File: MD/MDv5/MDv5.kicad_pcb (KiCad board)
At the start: 2 copper layers, 59.3 x 78.1 mm, 46 parts, among them J1 XT60PW-M, J2 XT60PW-M, J3 XT30PW-M, J4 XT30PW-M

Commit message: IRLB3813,L7805CV,L7812CV,74HC08N,78HC14NをSMDにして回路図完成
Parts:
- removed C1: 330μF, Capacitor_THT:CP_Radial_D8.0mm_P3.50mm
- removed C10, C11: 1.5μF, Library:C_Disc_D11.0mm_W5.0mm_P5.0mm_kai
- removed C2, C4, C6, C7, C8, C9: 0.1μF, Library:C_Disc_D11.0mm_W5.0mm_P5.0mm_kai
- removed C3, C5: 33μF, Capacitor_THT:CP_Radial_D5.0mm_P2.00mm
- removed D1: PWM_IN, LED_THT:LED_D5.0mm
- removed D2: 5V/2, LED_THT:LED_D5.0mm
- removed D3: 12V, LED_THT:LED_D5.0mm
- removed D4, D5: 1N4148DO35-7, Diode_THT:D_DO-35_SOD27_P7.62mm_Horizontal
- removed FET1, FET2, FET3, FET4: IRLB3813PBF, footprints:PG-TO220-3_INF
- removed IC1_NOT1, IC2_AND1: ~, Package_DIP:DIP-14_W7.62mm
- removed IC3, IC4, TLP2630: ~, Package_DIP:DIP-8_W7.62mm
- removed J1, J2: XT60PW-M, XT60-M:AMASS_XT60PW-M
- removed J3, J4: XT30PW-M, XT60-M:AMASS_XT30PW-M
- removed R1, R6, R7: 330Ω, Library:R_Axial_DIN0207_L6.3mm_D2.5mm_P10.16mm_Horizontal_kai
- removed R10, R11, R8, R9: 10kΩ, Library:R_Axial_DIN0207_L6.3mm_D2.5mm_P10.16mm_Horizontal_kai
- removed R2, R3, R4, R5: 200Ω, Library:R_Axial_DIN0207_L6.3mm_D2.5mm_P10.16mm_Horizontal_kai
- removed REF** (x4): MountingHole_3.2mm_M3, MountingHole:MountingHole_3.2mm_M3
- removed REFG5V1: L7805, footprints:PG-TO220-3_INF
- removed REG12V1: L7812, footprints:PG-TO220-3_INF
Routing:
- net +5V/2: track 126.3 -> 0.00 mm
- net GATE2: track 99.0 -> 0.00 mm, vias 4 -> 0
- net GND1: track 78.7 -> 0.00 mm, vias 1 -> 0
- net +12V: track 73.1 -> 0.00 mm
- net PWM_IN: track 67.8 -> 0.00 mm, vias 1 -> 0
- net GATE1: track 62.0 -> 0.00 mm
- net DIGITAL_IN: track 56.9 -> 0.00 mm, vias 1 -> 0
- net Net-(FET1-G): track 43.7 -> 0.00 mm, vias 2 -> 0
- net MOUT1: track 39.3 -> 0.00 mm, vias 2 -> 0
- net Net-(FET2-G): track 38.0 -> 0.00 mm, vias 6 -> 0
- net PWM_NOT: track 36.8 -> 0.00 mm, vias 3 -> 0
- net PWM1: track 31.6 -> 0.00 mm
- net Net-(D2-A): track 26.1 -> 0.00 mm
- net DIGITAL: track 25.7 -> 0.00 mm, vias 2 -> 0
- net DIGITAL_NOT: track 24.3 -> 0.00 mm, vias 1 -> 0
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- removed copper zone on B.Cu, net +24V
- removed copper zone on B.Cu, net GND2
- removed copper zone on F.Cu, net GND2
- removed copper zone on F.Cu, net MOUT1
- removed copper zone on F.Cu, net MOUT2
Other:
- board outline removed
- board text removed: "24V24V24V"
- board text removed: "DIGITAL_IN"
- board text removed: "GND1"
- board text removed: "GND2"
- board text removed: "MOUT1"
- board text removed: "MOUT2"
- board text removed: "PWM_IN"

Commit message: とりあえず配置
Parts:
- added C1: 330μF, Capacitor_THT:CP_Radial_D8.0mm_P3.50mm, F.Cu at (151.9, 100.6)
- added C10: 1.5μF, Library:C_Disc_D11.0mm_W5.0mm_P5.0mm_kai, F.Cu at (142.9, 77.2)
- added C11: 1.5μF, Library:C_Disc_D11.0mm_W5.0mm_P5.0mm_kai, F.Cu at (158.1, 76.9)
- added C2: 0.1μF, Library:C_Disc_D11.0mm_W5.0mm_P5.0mm_kai, F.Cu at (161.8, 106.7)
- added C3: 33μF, Capacitor_THT:CP_Radial_D5.0mm_P2.00mm, F.Cu at (162.9, 97.4)
- added C4: 0.1μF, Library:C_Disc_D11.0mm_W5.0mm_P5.0mm_kai, F.Cu at (151.2, 88.0)
- added C5: 33μF, Capacitor_THT:CP_Radial_D5.0mm_P2.00mm, F.Cu at (162.9, 90.9)
- added C6: 0.1μF, Library:C_Disc_D11.0mm_W5.0mm_P5.0mm_kai, F.Cu at (163.1, 86.0)
- added C7: 0.1μF, Library:C_Disc_D11.0mm_W5.0mm_P5.0mm_kai, F.Cu at (152.7, 69.3)
- added C8: 0.1μF, Library:C_Disc_D11.0mm_W5.0mm_P5.0mm_kai, F.Cu at (138.5, 69.3)
- added C9: 0.1μF, Library:C_Disc_D11.0mm_W5.0mm_P5.0mm_kai, F.Cu at (150.8, 53.7)
- added D1: PWM_IN, LED_THT:LED_D5.0mm, F.Cu at (124.4, 66.3)
- added D2: 5V/2, LED_THT:LED_D5.0mm, F.Cu at (160.3, 66.7)
- added D3: 12V, LED_THT:LED_D5.0mm, F.Cu at (160.3, 59.2)
- added D4: 1N4148W, Diode_SMD:D_SOD-123, F.Cu at (139.7, 75.4)
- added D5: 1N4148W, Diode_SMD:D_SOD-123, F.Cu at (154.6, 75.4)
- added FET1: RS6E120BGTB1, RS6G120BHTB1:RS6G120BHTB1, F.Cu at (143.9, 101.2)
- added FET2: RS6E120BGTB1, RS6G120BHTB1:RS6G120BHTB1, F.Cu at (134.7, 101.1)
- added FET3: RS6E120BGTB1, RS6G120BHTB1:RS6G120BHTB1, F.Cu at (143.7, 89.4)
- added FET4: RS6E120BGTB1, RS6G120BHTB1:RS6G120BHTB1, F.Cu at (134.7, 89.4)
- added IR2302S1: ~, Package_SO:SOIC-8_3.9x4.9mm_P1.27mm, F.Cu at (133.7, 75.6)
- added IR2302S2: ~, Package_SO:SOIC-8_3.9x4.9mm_P1.27mm, F.Cu at (148.8, 75.6)
- added J1: XT60PW-M, XT60PW-M:AMASS_XT60PW-M, F.Cu at (151.8, 113.8)
- added J2: XT60PW-M, XT60PW-M:AMASS_XT60PW-M, F.Cu at (134.7, 113.8)
- added J3: XT30PW-M, Connector_AMASS:AMASS_XT30PW-M_1x02_P2.50mm_Horizontal, F.Cu at (126.6, 94.8)
- added J4: XT30PW-M, Connector_AMASS:AMASS_XT30PW-M_1x02_P2.50mm_Horizontal, F.Cu at (126.6, 79.5)
- added R1: 330Ω, Capacitor_SMD:C_0805_2012Metric, F.Cu at (127.6, 58.2)
- added R10: 10kΩ, Capacitor_SMD:C_0805_2012Metric, F.Cu at (143.7, 80.8)
- added R11: 10kΩ, Capacitor_SMD:C_0805_2012Metric, F.Cu at (134.7, 80.8)
- added R2: 200Ω, Capacitor_SMD:C_0805_2012Metric, F.Cu at (164.0, 76.1)
- added R3: 200Ω, Capacitor_SMD:C_0805_2012Metric, F.Cu at (161.0, 76.1)
- added R4: 120Ω, Capacitor_SMD:C_0805_2012Metric, F.Cu at (133.9, 57.1)
- added R5: 200Ω, Capacitor_SMD:C_0805_2012Metric, F.Cu at (133.9, 60.3)
- added R6: 330Ω, Capacitor_SMD:C_0805_2012Metric, F.Cu at (152.9, 57.1)
- added R7: 330Ω, Capacitor_SMD:C_0805_2012Metric, F.Cu at (152.9, 60.2)
- added R8: 10kΩ, Capacitor_SMD:C_0805_2012Metric, F.Cu at (143.9, 92.6)
- added R9: 10kΩ, Capacitor_SMD:C_0805_2012Metric, F.Cu at (134.7, 92.6)
- added REF1: MountingHole_3.2mm_M3, MountingHole:MountingHole_3.2mm_M3, F.Cu at (119.0, 55.0)
- added REF2: MountingHole_3.2mm_M3, MountingHole:MountingHole_3.2mm_M3, F.Cu at (166.0, 55.0)
- added REF3: MountingHole_3.2mm_M3, MountingHole:MountingHole_3.2mm_M3, F.Cu at (166.0, 117.0)
- added REF4: MountingHole_3.2mm_M3, MountingHole:MountingHole_3.2mm_M3, F.Cu at (119.0, 117.0)
- added REFG5V1: MC7805CDTG, footprints:PG-TO220-3_INF, F.Cu at (151.2, 83.9)
- added REG12V1: L7812CD2T-TR, footprints:PG-TO220-3_INF, F.Cu at (151.2, 93.1)
- added TC74HC08AF1: ~, Package_SO:SOIC-14_3.9x8.7mm_P1.27mm, F.Cu at (131.9, 66.8)
- added TC74HC14AF1: ~, Package_SO:SOIC-14_3.9x8.7mm_P1.27mm, F.Cu at (146.0, 66.7)
- added TLP2630: ~, Package_DIP:DIP-8_W7.62mm, F.Cu at (139.6, 53.1)
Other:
- board outline added: 55 x 70 mm
- board text added: "DIGITAL_IN"
- board text added: "GND1"
- board text added: "PWM_IN"

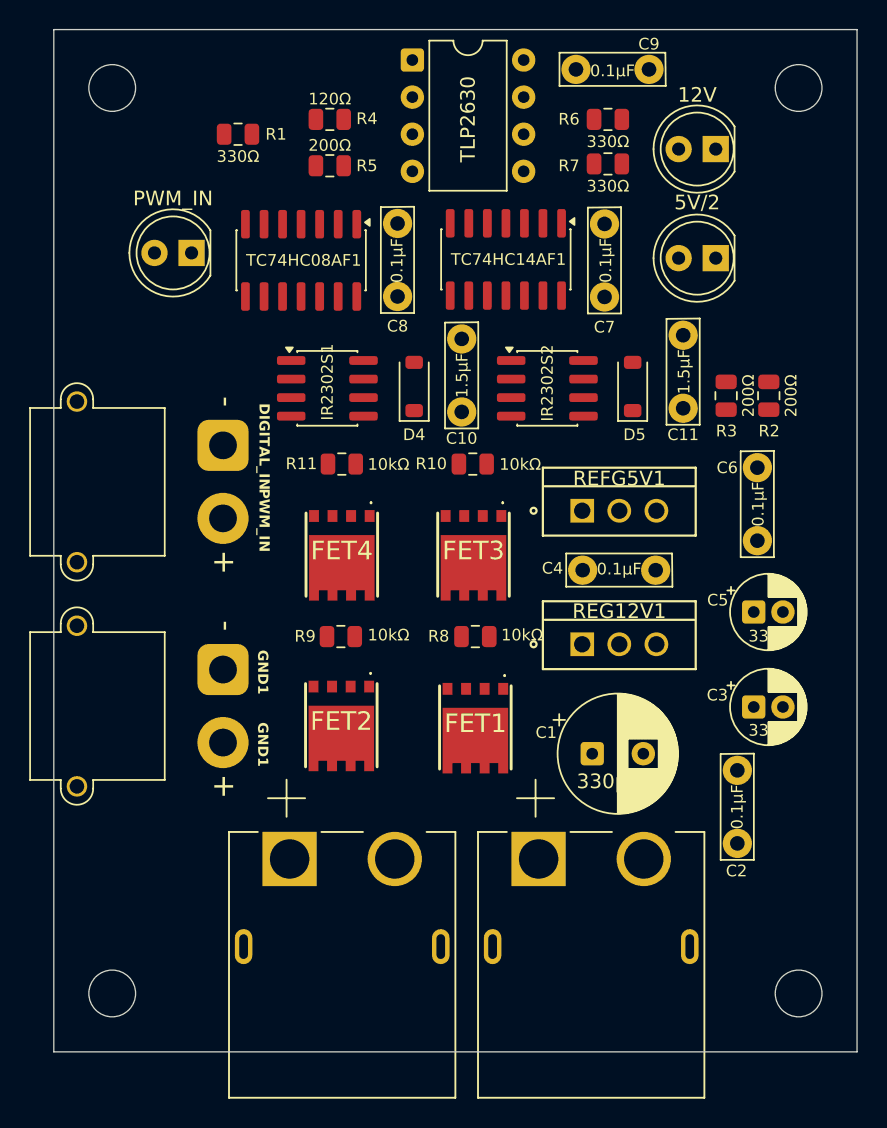
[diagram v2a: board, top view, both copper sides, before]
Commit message: ちょっと変えた
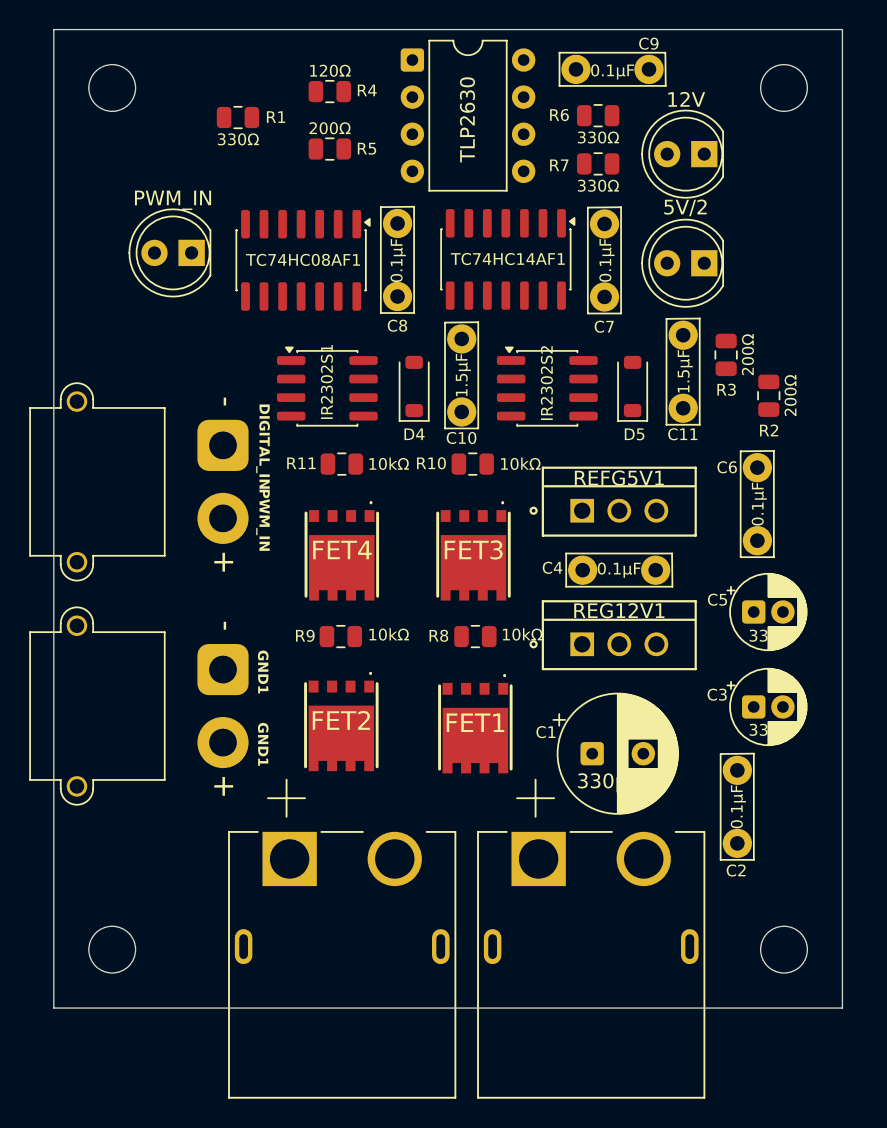
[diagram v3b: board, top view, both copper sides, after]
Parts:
- moved REF3 3.16 mm to (165.0, 114.0)
- moved REF4 3.00 mm to (119.0, 114.0)
- moved R3 2.79 mm to (161.0, 73.3)
- moved R4 1.91 mm to (133.9, 55.2)
- moved R5 1.14 mm to (133.9, 59.2)
- moved R1 1.14 mm to (127.6, 57.0)
- moved REF2 1.00 mm to (165.0, 55.0)
- moved D2 0.86 mm to (159.5, 67.0)
- moved D3 0.86 mm to (159.5, 59.5)
- moved R6 0.72 mm to (152.3, 56.9)
- moved R7 0.67 mm to (152.3, 60.2)
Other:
- board size 55 x 70 mm -> 54 x 67 mm
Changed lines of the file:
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@@
 	(footprint "MountingHole:MountingHole_3.2mm_M3"
 		(layer "F.Cu")
-		(at 119 117)
+		(at 119 114)
 		(descr "Mounting Hole 3.2mm, M3, no annular, generated by kicad-footprint-generator mountinghole.py")
 		(tags "mountinghole M3")
@@
 	(footprint "Capacitor_SMD:C_0805_2012Metric"
 		(layer "F.Cu")
-		(at 127.6146 58.166)
+		(at 127.6146 57.023)
 		(descr "Capacitor SMD 0805 (2012 Metric), square (rectangular) end terminal, IPC-7351 nominal, (Body size source: IPC-SM-782 page 76, https://www.pcb-3d.com/wordpress/wp-content/uploads/ipc-sm-782a_amendment_1_and_2.pdf, https://docs.google.com/spreadsheets/d/1BsfQQcO9C6DZCsRaXUlFlo91Tg2WpOkGARC1WS5S8t0/edit?usp=sharing), generated with kicad-footprint-generator")
 		(tags "capacitor")
@@
 	(footprint "MountingHole:MountingHole_3.2mm_M3"
 		(layer "F.Cu")
-		(at 166 117)
+		(at 165 114)
 		(descr "Mounting Hole 3.2mm, M3, no annular, generated by kicad-footprint-generator mountinghole.py")
 		(tags "mountinghole M3")
@@
 	(footprint "Capacitor_SMD:C_0805_2012Metric"
 		(layer "F.Cu")
-		(at 161.036 76.073 90)
+		(at 161.036 73.279 90)
 		(descr "Capacitor SMD 0805 (2012 Metric), square (rectangular) end terminal, IPC-7351 nominal, (Body size source: IPC-SM-782 page 76, https://www.pcb-3d.com/wordpress/wp-content/uploads/ipc-sm-782a_amendment_1_and_2.pdf, https://docs.google.com/spreadsheets/d/1BsfQQcO9C6DZCsRaXUlFlo91Tg2WpOkGARC1WS5S8t0/edit?usp=sharing), generated with kicad-footprint-generator")
 		(tags "capacitor")
@@
 	(footprint "LED_THT:LED_D5.0mm"
 		(layer "F.Cu")
-		(at 160.3248 66.652 180)
+		(at 159.54 67 180)
 		(descr "LED, diameter 5.0mm, 2 pins, http://cdn-reichelt.de/documents/datenblatt/A500/LL-504BC2E-009.pdf, generated by kicad-footprint-generator")
 		(tags "LED")
@@
 	(footprint "Capacitor_SMD:C_0805_2012Metric"
 		(layer "F.Cu")
-		(at 133.8986 60.325 180)
+		(at 133.8986 59.182 180)
 		(descr "Capacitor SMD 0805 (2012 Metric), square (rectangular) end terminal, IPC-7351 nominal, (Body size source: IPC-SM-782 page 76, https://www.pcb-3d.com/wordpress/wp-content/uploads/ipc-sm-782a_amendment_1_and_2.pdf, https://docs.google.com/spreadsheets/d/1BsfQQcO9C6DZCsRaXUlFlo91Tg2WpOkGARC1WS5S8t0/edit?usp=sharing), generated with kicad-footprint-generator")
 		(tags "capacitor")
@@
 	(footprint "Capacitor_SMD:C_0805_2012Metric"
 		(layer "F.Cu")
-		(at 152.9436 60.198)
+		(at 152.273 60.198)
 		(descr "Capacitor SMD 0805 (2012 Metric), square (rectangular) end terminal, IPC-7351 nominal, (Body size source: IPC-SM-782 page 76, https://www.pcb-3d.com/wordpress/wp-content/uploads/ipc-sm-782a_amendment_1_and_2.pdf, https://docs.google.com/spreadsheets/d/1BsfQQcO9C6DZCsRaXUlFlo91Tg2WpOkGARC1WS5S8t0/edit?usp=sharing), generated with kicad-footprint-generator")
 		(tags "capacitor")
@@
 	(footprint "LED_THT:LED_D5.0mm"
 		(layer "F.Cu")
-		(at 160.3248 59.182 180)
+		(at 159.54 59.53 180)
 		(descr "LED, diameter 5.0mm, 2 pins, http://cdn-reichelt.de/documents/datenblatt/A500/LL-504BC2E-009.pdf, generated by kicad-footprint-generator")
 		(tags "LED")
@@
 	(footprint "MountingHole:MountingHole_3.2mm_M3"
 		(layer "F.Cu")
-		(at 166 55)
+		(at 165 55)
 		(descr "Mounting Hole 3.2mm, M3, no annular, generated by kicad-footprint-generator mountinghole.py")
 		(tags "mountinghole M3")
@@
 	(footprint "Capacitor_SMD:C_0805_2012Metric"
 		(layer "F.Cu")
-		(at 152.9436 57.15)
+		(at 152.273 56.896)
 		(descr "Capacitor SMD 0805 (2012 Metric), square (rectangular) end terminal, IPC-7351 nominal, (Body size source: IPC-SM-782 page 76, https://www.pcb-3d.com/wordpress/wp-content/uploads/ipc-sm-782a_amendment_1_and_2.pdf, https://docs.google.com/spreadsheets/d/1BsfQQcO9C6DZCsRaXUlFlo91Tg2WpOkGARC1WS5S8t0/edit?usp=sharing), generated with kicad-footprint-generator")
 		(tags "capacitor")
@@
 	(footprint "Capacitor_SMD:C_0805_2012Metric"
 		(layer "F.Cu")
-		(at 133.8986 57.15 180)
+		(at 133.8986 55.245 180)
 		(descr "Capacitor SMD 0805 (2012 Metric), square (rectangular) end terminal, IPC-7351 nominal, (Body size source: IPC-SM-782 page 76, https://www.pcb-3d.com/wordpress/wp-content/uploads/ipc-sm-782a_amendment_1_and_2.pdf, https://docs.google.com/spreadsheets/d/1BsfQQcO9C6DZCsRaXUlFlo91Tg2WpOkGARC1WS5S8t0/edit?usp=sharing), generated with kicad-footprint-generator")
 		(tags "capacitor")
@@
 	(gr_rect
 		(start 115 51)
-		(end 170 121)
+		(end 169 118)
 		(stroke
 			(width 0.05)
